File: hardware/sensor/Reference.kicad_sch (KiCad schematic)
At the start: 3 parts

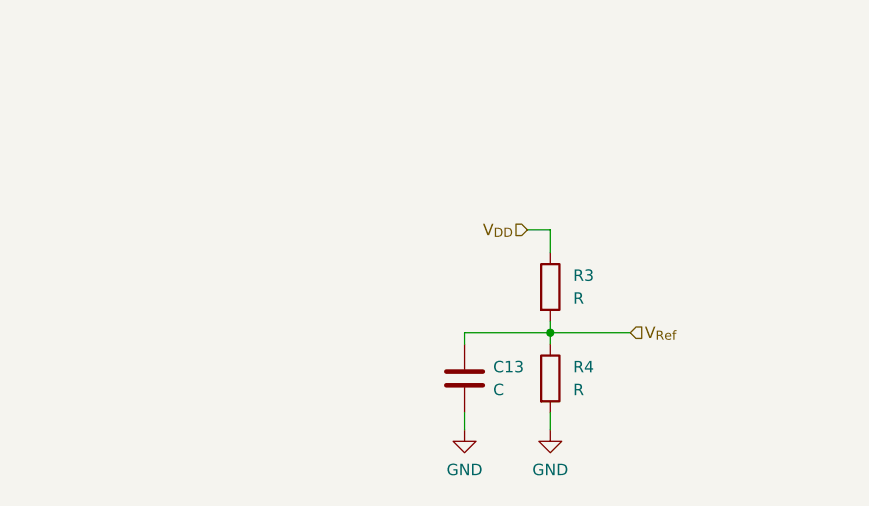
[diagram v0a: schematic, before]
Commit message: commit to save work from misbehaving laptop
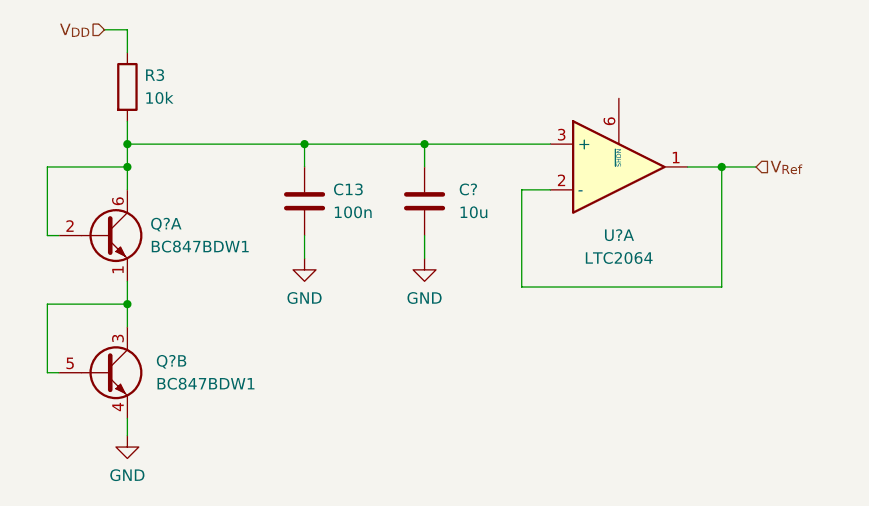
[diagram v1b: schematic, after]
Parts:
- removed R4: R, symbol Device:R
- added C?: 10u, symbol Device:C
- added Q? (x2): BC847BDW1, Package_TO_SOT_SMD:SOT-363_SC-70-6, symbol Transistor_BJT:BC847BDW1
- added U?: LTC2064, Package_SO:MSOP-8_3x3mm_P0.65mm, symbol sensorModules:LTC2064IMS8
- C13: value C -> 100n
- R3: value R -> 10k
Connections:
- net GND: now also C?.2, Q?.4 (E2)
- net V_{Ref}: now also U?.1, U?.2 (-); no longer C13.1, R3.2
- new net: Q?.1 (E1), Q?.3 (C2), Q?.5 (B2)
- new net: C13.1, C?.1, Q?.2 (B1), Q?.6 (C1), R3.2, U?.3 (+)
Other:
- moved on the sheet: C13, R3
